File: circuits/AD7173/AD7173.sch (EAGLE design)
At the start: 35 parts, among them IC1 AD7173, IC2 ADP1720, IC3 ADP1720ARMZ-5, IC4 ADR445BR, Q1 FA-20H

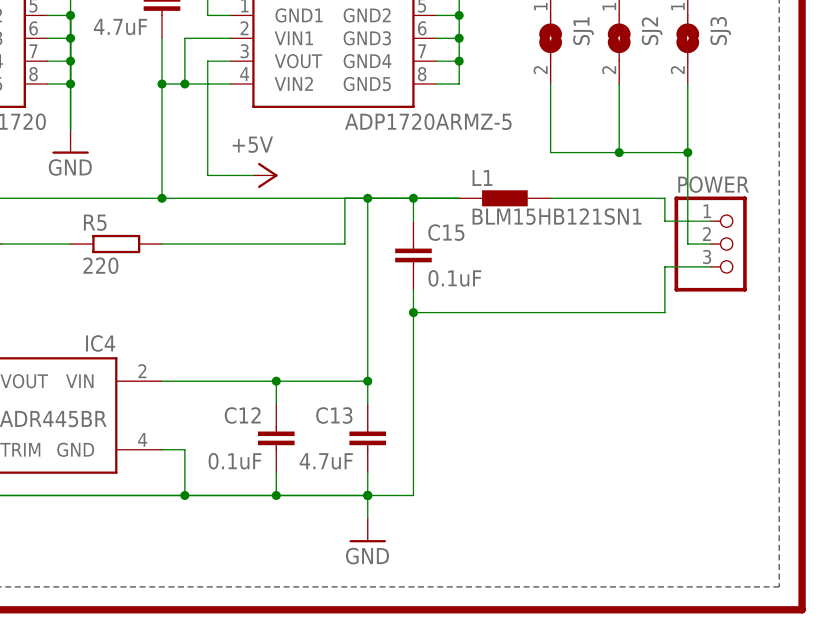
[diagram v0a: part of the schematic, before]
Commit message: upadted AD7173 breakout board
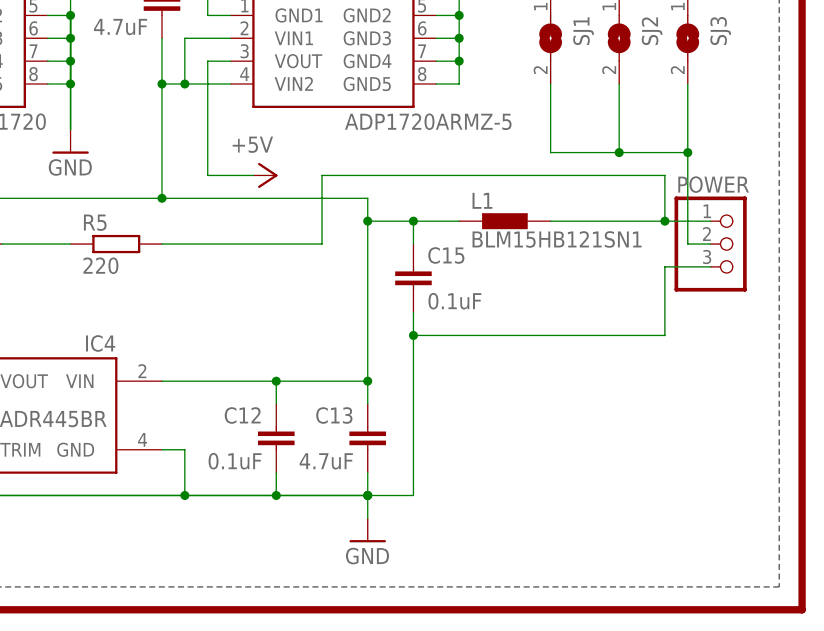
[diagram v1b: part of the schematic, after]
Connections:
- net N$30: now also R5.2
- net VIN: no longer R5.2
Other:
- moved on the sheet: C15, L1
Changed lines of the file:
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@@
 <instance part="P+2" gate="VCC" x="127" y="96.52"/>
 <instance part="P+1" gate="VCC" x="162.56" y="35.56"/>
-<instance part="L1" gate="G$1" x="241.3" y="45.72"/>
-<instance part="C15" gate="G$1" x="231.14" y="40.64"/>
+<instance part="L1" gate="G$1" x="241.3" y="43.18"/>
+<instance part="C15" gate="G$1" x="231.14" y="38.1"/>
 <instance part="P+4" gate="1" x="12.7" y="99.06"/>
 <instance part="SJ1" gate="1" x="246.38" y="63.5" rot="R270"/>
@@
 <pinref part="GND5" gate="1" pin="GND"/>
 <wire x1="226.06" y1="12.7" x2="231.14" y2="12.7" width="0.1524" layer="91"/>
-<wire x1="231.14" y1="12.7" x2="231.14" y2="33.02" width="0.1524" layer="91"/>
+<wire x1="231.14" y1="12.7" x2="231.14" y2="30.48" width="0.1524" layer="91"/>
 <pinref part="IC4" gate="G$1" pin="GND"/>
 <pinref part="C11" gate="G$1" pin="2"/>
@@
 <wire x1="162.56" y1="12.7" x2="172.72" y2="12.7" width="0.1524" layer="91"/>
 <wire x1="172.72" y1="12.7" x2="172.72" y2="15.24" width="0.1524" layer="91"/>
-<junction x="231.14" y="33.02"/>
+<junction x="231.14" y="30.48"/>
 <wire x1="264.16" y1="38.1" x2="259.08" y2="38.1" width="0.1524" layer="91"/>
-<wire x1="259.08" y1="38.1" x2="259.08" y2="33.02" width="0.1524" layer="91"/>
+<wire x1="259.08" y1="38.1" x2="259.08" y2="30.48" width="0.1524" layer="91"/>
 <pinref part="C15" gate="G$1" pin="2"/>
-<wire x1="259.08" y1="33.02" x2="231.14" y2="33.02" width="0.1524" layer="91"/>
-<wire x1="231.14" y1="33.02" x2="231.14" y2="35.56" width="0.1524" layer="91"/>
+<wire x1="259.08" y1="30.48" x2="231.14" y2="30.48" width="0.1524" layer="91"/>
+<wire x1="231.14" y1="30.48" x2="231.14" y2="33.02" width="0.1524" layer="91"/>
 <junction x="172.72" y="12.7"/>
 <pinref part="LED2" gate="G$1" pin="C"/>
@@
 <pinref part="C3" gate="G$1" pin="2"/>
 <wire x1="160.02" y1="63.5" x2="160.02" y2="58.42" width="0.1524" layer="91"/>
+<wire x1="226.06" y1="43.18" x2="226.06" y2="45.72" width="0.1524" layer="91"/>
 <wire x1="226.06" y1="45.72" x2="203.2" y2="45.72" width="0.1524" layer="91"/>
 <wire x1="203.2" y1="45.72" x2="160.02" y2="45.72" width="0.1524" layer="91"/>
@@
 <junction x="162.56" y="58.42"/>
 <junction x="203.2" y="58.42"/>
-<wire x1="226.06" y1="25.4" x2="226.06" y2="45.72" width="0.1524" layer="91"/>
+<wire x1="226.06" y1="25.4" x2="226.06" y2="43.18" width="0.1524" layer="91"/>
 <pinref part="C13" gate="G$1" pin="1"/>
 <junction x="226.06" y="25.4"/>
 <junction x="215.9" y="25.4"/>
 <pinref part="L1" gate="G$1" pin="1"/>
-<wire x1="231.14" y1="45.72" x2="226.06" y2="45.72" width="0.1524" layer="91"/>
+<wire x1="231.14" y1="43.18" x2="226.06" y2="43.18" width="0.1524" layer="91"/>
 <wire x1="226.06" y1="25.4" x2="226.06" y2="22.86" width="0.1524" layer="91"/>
 <pinref part="C15" gate="G$1" pin="1"/>
-<wire x1="236.22" y1="45.72" x2="231.14" y2="45.72" width="0.1524" layer="91"/>
-<wire x1="231.14" y1="45.72" x2="231.14" y2="43.18" width="0.1524" layer="91"/>
-<junction x="226.06" y="45.72"/>
-<junction x="231.14" y="45.72"/>
-<wire x1="236.22" y1="45.72" x2="223.52" y2="45.72" width="0.1524" layer="91"/>
-<wire x1="223.52" y1="45.72" x2="223.52" y2="40.64" width="0.1524" layer="91"/>
-<pinref part="R5" gate="G$1" pin="2"/>
-<wire x1="223.52" y1="40.64" x2="203.2" y2="40.64" width="0.1524" layer="91"/>
+<wire x1="236.22" y1="43.18" x2="231.14" y2="43.18" width="0.1524" layer="91"/>
+<wire x1="231.14" y1="43.18" x2="231.14" y2="40.64" width="0.1524" layer="91"/>
+<junction x="226.06" y="43.18"/>
+<junction x="231.14" y="43.18"/>
 </segment>
 </net>
@@
 <pinref part="L1" gate="G$1" pin="2"/>
 <wire x1="264.16" y1="43.18" x2="259.08" y2="43.18" width="0.1524" layer="91"/>
-<wire x1="259.08" y1="43.18" x2="259.08" y2="45.72" width="0.1524" layer="91"/>
-<wire x1="259.08" y1="45.72" x2="246.38" y2="45.72" width="0.1524" layer="91"/>
-</segment>
-</net>
+<wire x1="259.08" y1="43.18" x2="246.38" y2="43.18" width="0.1524" layer="91"/>
+<wire x1="259.08" y1="43.18" x2="259.08" y2="48.26" width="0.1524" layer="91"/>
+<wire x1="259.08" y1="48.26" x2="220.98" y2="48.26" width="0.1524" layer="91"/>
+<wire x1="220.98" y1="48.26" x2="220.98" y2="40.64" width="0.1524" layer="91"/>
+<pinref part="R5" gate="G$1" pin="2"/>
+<wire x1="220.98" y1="40.64" x2="203.2" y2="40.64" width="0.1524" layer="91"/>
+<junction x="259.08" y="43.18"/>
+</segment>
+</net>

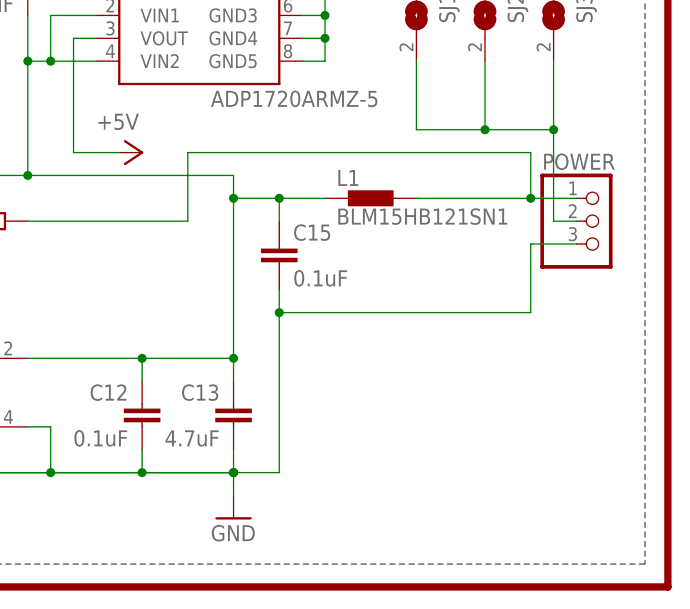
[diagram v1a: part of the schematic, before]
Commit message: upadted AD7173 breakout board
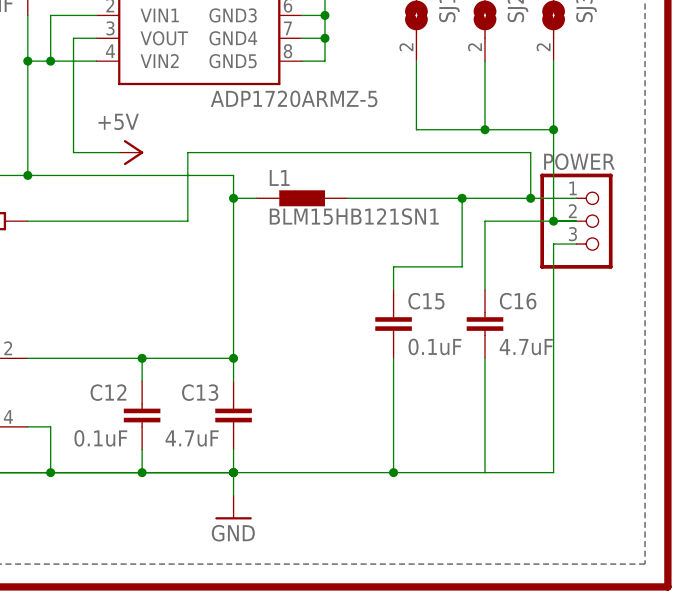
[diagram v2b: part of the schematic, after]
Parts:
- added C16: 4.7uF, rcl:C-EUC0402
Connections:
- net GND: now also C16.2
- net N$28: now also C16.1
- net N$30: now also C15.1
- net VIN: no longer C15.1
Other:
- moved on the sheet: C15, L1
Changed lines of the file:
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@@
 <part name="LED2" library="led" deviceset="LED" device="CHIP-LED0603"/>
 <part name="R5" library="rcl" deviceset="R-EU_" device="R0402" value="220"/>
+<part name="C16" library="rcl" deviceset="C-EU" device="C0402" value="4.7uF"/>
 </parts>
 <sheets>
@@
 <instance part="P+2" gate="VCC" x="127" y="96.52"/>
 <instance part="P+1" gate="VCC" x="162.56" y="35.56"/>
-<instance part="L1" gate="G$1" x="241.3" y="43.18"/>
-<instance part="C15" gate="G$1" x="231.14" y="38.1"/>
+<instance part="L1" gate="G$1" x="233.68" y="43.18"/>
+<instance part="C15" gate="G$1" x="243.84" y="30.48"/>
 <instance part="P+4" gate="1" x="12.7" y="99.06"/>
 <instance part="SJ1" gate="1" x="246.38" y="63.5" rot="R270"/>
@@
 <instance part="LED2" gate="G$1" x="182.88" y="40.64" rot="R270"/>
 <instance part="R5" gate="G$1" x="198.12" y="40.64"/>
+<instance part="C16" gate="G$1" x="254" y="30.48"/>
 </instances>
 <busses>
@@
 <pinref part="POWER" gate="A" pin="3"/>
 <pinref part="GND5" gate="1" pin="GND"/>
-<wire x1="226.06" y1="12.7" x2="231.14" y2="12.7" width="0.1524" layer="91"/>
-<wire x1="231.14" y1="12.7" x2="231.14" y2="30.48" width="0.1524" layer="91"/>
+<wire x1="226.06" y1="12.7" x2="243.84" y2="12.7" width="0.1524" layer="91"/>
 <pinref part="IC4" gate="G$1" pin="GND"/>
 <pinref part="C11" gate="G$1" pin="2"/>
@@
 <wire x1="162.56" y1="12.7" x2="172.72" y2="12.7" width="0.1524" layer="91"/>
 <wire x1="172.72" y1="12.7" x2="172.72" y2="15.24" width="0.1524" layer="91"/>
-<junction x="231.14" y="30.48"/>
-<wire x1="264.16" y1="38.1" x2="259.08" y2="38.1" width="0.1524" layer="91"/>
-<wire x1="259.08" y1="38.1" x2="259.08" y2="30.48" width="0.1524" layer="91"/>
+<junction x="243.84" y="12.7"/>
 <pinref part="C15" gate="G$1" pin="2"/>
-<wire x1="259.08" y1="30.48" x2="231.14" y2="30.48" width="0.1524" layer="91"/>
-<wire x1="231.14" y1="30.48" x2="231.14" y2="33.02" width="0.1524" layer="91"/>
+<wire x1="254" y1="12.7" x2="243.84" y2="12.7" width="0.1524" layer="91"/>
+<wire x1="243.84" y1="12.7" x2="243.84" y2="25.4" width="0.1524" layer="91"/>
 <junction x="172.72" y="12.7"/>
 <pinref part="LED2" gate="G$1" pin="C"/>
@@
 <wire x1="226.06" y1="12.7" x2="226.06" y2="10.16" width="0.1524" layer="91"/>
 <junction x="162.56" y="12.7"/>
+<pinref part="C16" gate="G$1" pin="2"/>
+<wire x1="254" y1="25.4" x2="254" y2="12.7" width="0.1524" layer="91"/>
+<wire x1="254" y1="12.7" x2="261.62" y2="12.7" width="0.1524" layer="91"/>
+<wire x1="261.62" y1="12.7" x2="261.62" y2="38.1" width="0.1524" layer="91"/>
+<wire x1="261.62" y1="38.1" x2="264.16" y2="38.1" width="0.1524" layer="91"/>
 </segment>
 <segment>
@@
 <junction x="215.9" y="25.4"/>
 <pinref part="L1" gate="G$1" pin="1"/>
-<wire x1="231.14" y1="43.18" x2="226.06" y2="43.18" width="0.1524" layer="91"/>
 <wire x1="226.06" y1="25.4" x2="226.06" y2="22.86" width="0.1524" layer="91"/>
-<pinref part="C15" gate="G$1" pin="1"/>
-<wire x1="236.22" y1="43.18" x2="231.14" y2="43.18" width="0.1524" layer="91"/>
-<wire x1="231.14" y1="43.18" x2="231.14" y2="40.64" width="0.1524" layer="91"/>
+<wire x1="228.6" y1="43.18" x2="226.06" y2="43.18" width="0.1524" layer="91"/>
 <junction x="226.06" y="43.18"/>
-<junction x="231.14" y="43.18"/>
 </segment>
 </net>
@@
 <pinref part="POWER" gate="A" pin="1"/>
 <pinref part="L1" gate="G$1" pin="2"/>
-<wire x1="264.16" y1="43.18" x2="259.08" y2="43.18" width="0.1524" layer="91"/>
-<wire x1="259.08" y1="43.18" x2="246.38" y2="43.18" width="0.1524" layer="91"/>
+<wire x1="259.08" y1="43.18" x2="251.46" y2="43.18" width="0.1524" layer="91"/>
+<wire x1="251.46" y1="43.18" x2="238.76" y2="43.18" width="0.1524" layer="91"/>
 <wire x1="259.08" y1="43.18" x2="259.08" y2="48.26" width="0.1524" layer="91"/>
 <wire x1="259.08" y1="48.26" x2="220.98" y2="48.26" width="0.1524" layer="91"/>
@@
 <wire x1="220.98" y1="40.64" x2="203.2" y2="40.64" width="0.1524" layer="91"/>
 <junction x="259.08" y="43.18"/>
+<pinref part="C15" gate="G$1" pin="1"/>
+<wire x1="243.84" y1="33.02" x2="243.84" y2="35.56" width="0.1524" layer="91"/>
+<wire x1="243.84" y1="35.56" x2="251.46" y2="35.56" width="0.1524" layer="91"/>
+<wire x1="251.46" y1="35.56" x2="251.46" y2="43.18" width="0.1524" layer="91"/>
+<wire x1="259.08" y1="43.18" x2="264.16" y2="43.18" width="0.1524" layer="91"/>
+<junction x="251.46" y="43.18"/>
 </segment>
 </net>
@@
 <junction x="261.62" y="50.8"/>
 <junction x="254" y="50.8"/>
-</segment>
-</net>
+<pinref part="C16" gate="G$1" pin="1"/>
+<wire x1="264.16" y1="40.64" x2="261.62" y2="40.64" width="0.1524" layer="91"/>
+<wire x1="261.62" y1="40.64" x2="254" y2="40.64" width="0.1524" layer="91"/>
+<wire x1="254" y1="40.64" x2="254" y2="33.02" width="0.1524" layer="91"/>
+<junction x="261.62" y="40.64"/>
+</segment>
+</net>
